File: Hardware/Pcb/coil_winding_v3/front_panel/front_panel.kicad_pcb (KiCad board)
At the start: 2 copper layers, 180.9 x 83.4 mm, 17 parts, among them J1 Conn_01x14_Socket, J4 Conn_01x13_Socket, SW1 SW_Push, SW2 SW_Push, SW3 RotaryEncoder_Switch

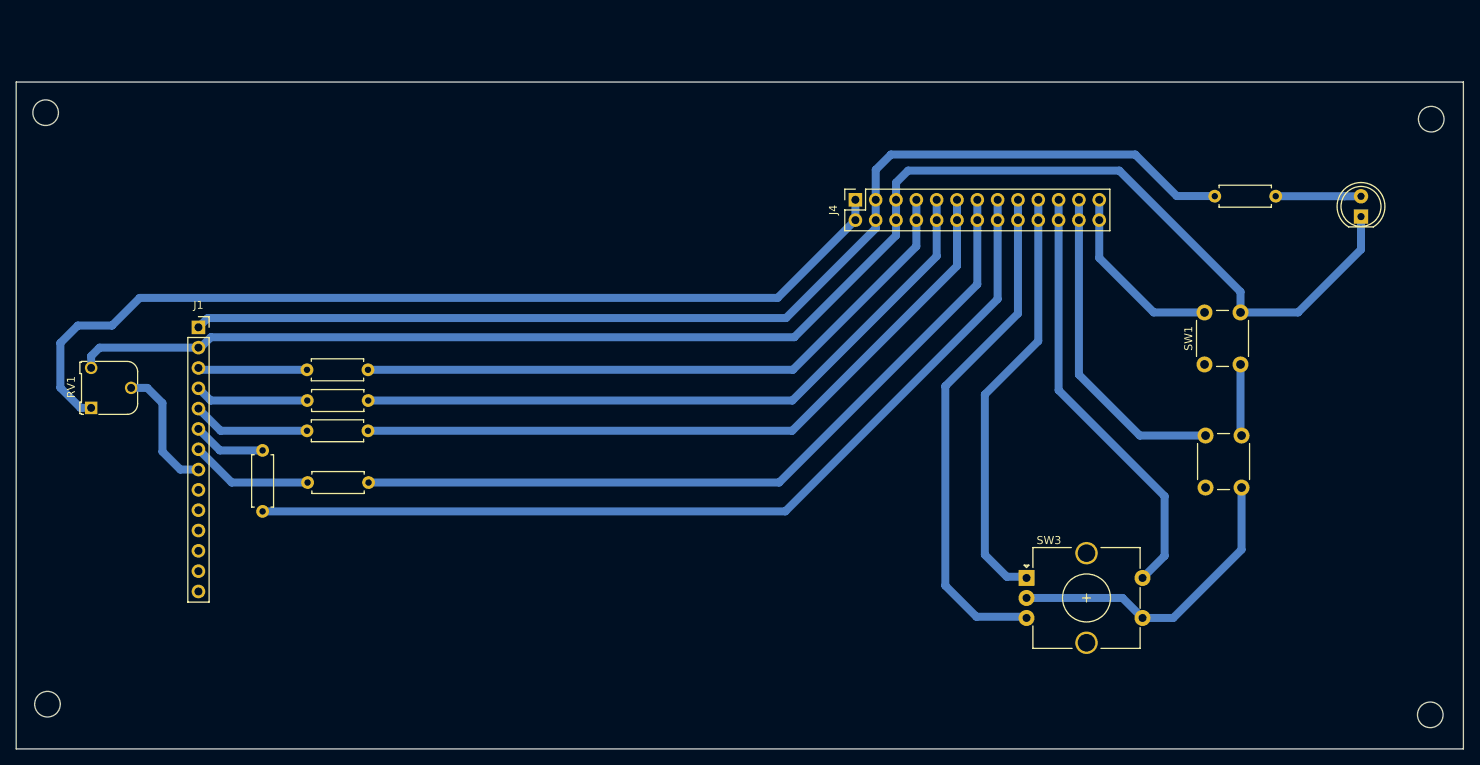
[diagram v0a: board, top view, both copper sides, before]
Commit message: final_code
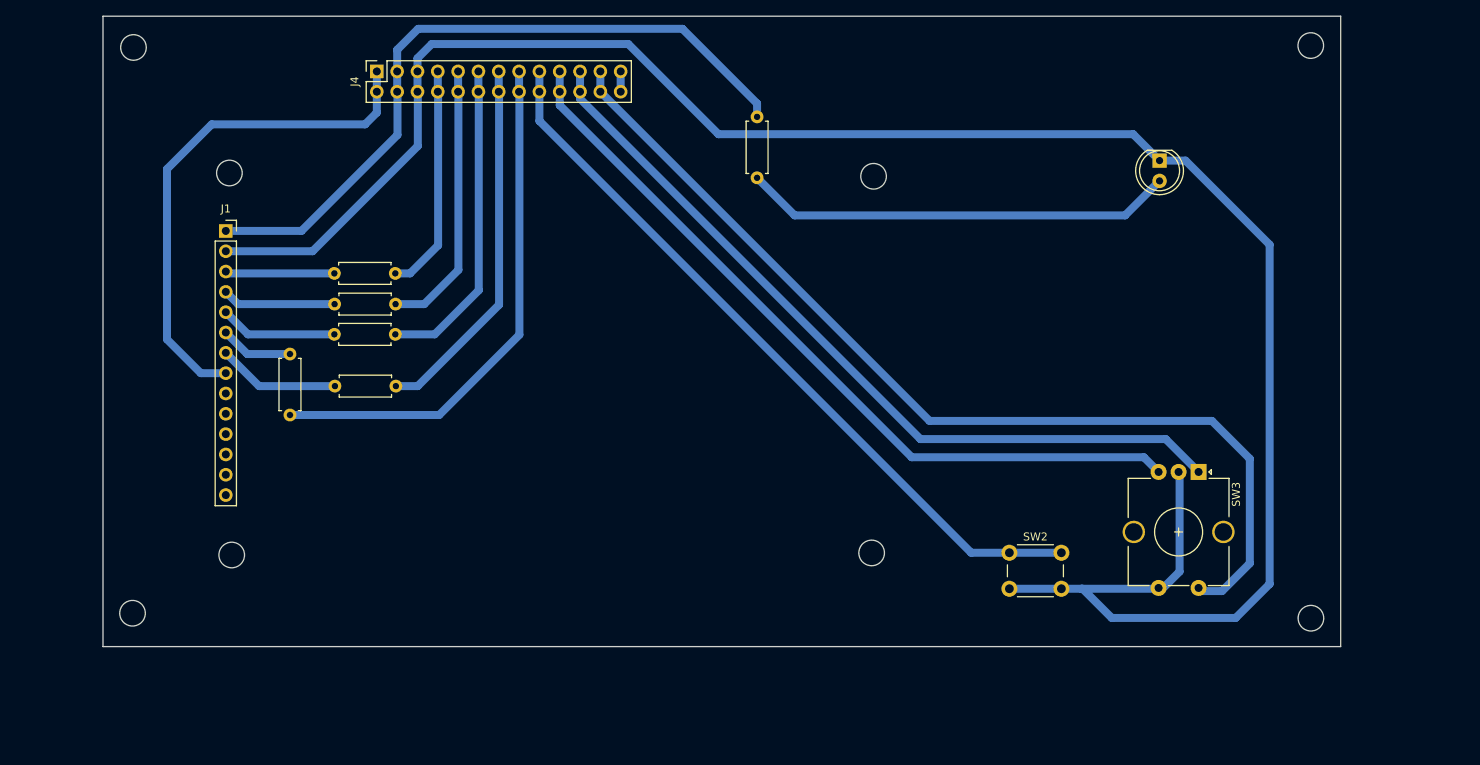
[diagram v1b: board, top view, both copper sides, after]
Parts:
- removed RV1: R_Potentiometer, Potentiometer_THT:Potentiometer_Runtron_RM-065_Vertical
- removed SW1: SW_Push, Button_Switch_THT:SW_PUSH_6mm_H7.3mm
- added H1: MountingHole, MountingHole:MountingHole_3.2mm_M3, F.Cu at (145.4, 104.0)
- added H1: MountingHole, MountingHole:MountingHole_3.2mm_M3, F.Cu at (145.6, 56.9)
- added H1: MountingHole, MountingHole:MountingHole_3.2mm_M3, F.Cu at (65.4, 104.2)
- added H1: MountingHole, MountingHole:MountingHole_3.2mm_M3, F.Cu at (65.1, 56.5)
- moved J4 61.9 mm to (83.5, 43.8)
- moved R1 58.1 mm to (131.1, 49.5), turned to -90 degrees
- moved D1 26.1 mm to (181.4, 54.9), turned to -90 degrees
- moved SW2 25.8 mm to (162.6, 103.9), turned to 0 degrees
- moved SW3 25.3 mm to (186.3, 93.8), turned to -90 degrees
- moved H3 19.2 mm to (200.3, 112.1)
- moved H4 17.6 mm to (200.3, 40.5)
- moved H2 15.6 mm to (53.0, 111.5)
- moved H1 13.7 mm to (53.1, 40.8)
- moved R7 12.5 mm to (72.7, 79.1)
- moved J1 12.5 mm to (64.7, 63.7)
- moved R2 12.5 mm to (78.2, 69.0)
- moved R3 12.5 mm to (78.3, 72.9)
- moved R4 12.5 mm to (78.2, 76.6)
- moved R6 12.5 mm to (78.3, 83.1)
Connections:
- J1 pad 8: Net-(J1-Pin_8) -> +3V3
- J4 pad 10: D2 -> D3
- J4 pad 11: D4 -> D2
- J4 pad 12: D7 -> D4
- J4 pad 13: D8 -> unconnected-(J4-Pin_13-Pad13)
- J4 pad 9: D3 -> D7
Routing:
- net D4: track 53.9 -> 123.4 mm
- net +3V3: track 118.8 -> 64.7 mm
- net +5V: track 142.6 -> 88.8 mm
- net D7: track 40.8 -> 94.3 mm
- net A5: track 80.8 -> 28.6 mm
- net A4: track 85.6 -> 34.5 mm
- net D13: track 96.9 -> 46.3 mm
- net A3: track 90.4 -> 40.1 mm
- net D11: track 115.3 -> 65.8 mm
- net D2: track 53.5 -> 100.1 mm
- net Net-(D1-A): track 10.7 -> 54.0 mm
- net D3: track 63.8 -> 98.1 mm
- net GND: track 238.2 -> 262.4 mm
- net D8: track 23.3 -> 0.00 mm
- net Net-(J1-Pin_8): track 16.2 -> 0.00 mm
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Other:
- board size 180.9 x 83.4 mm -> 154.7 x 78.8 mm
